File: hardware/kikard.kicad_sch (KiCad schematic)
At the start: 1 part, among them U1 NRF52840-QIAA-R

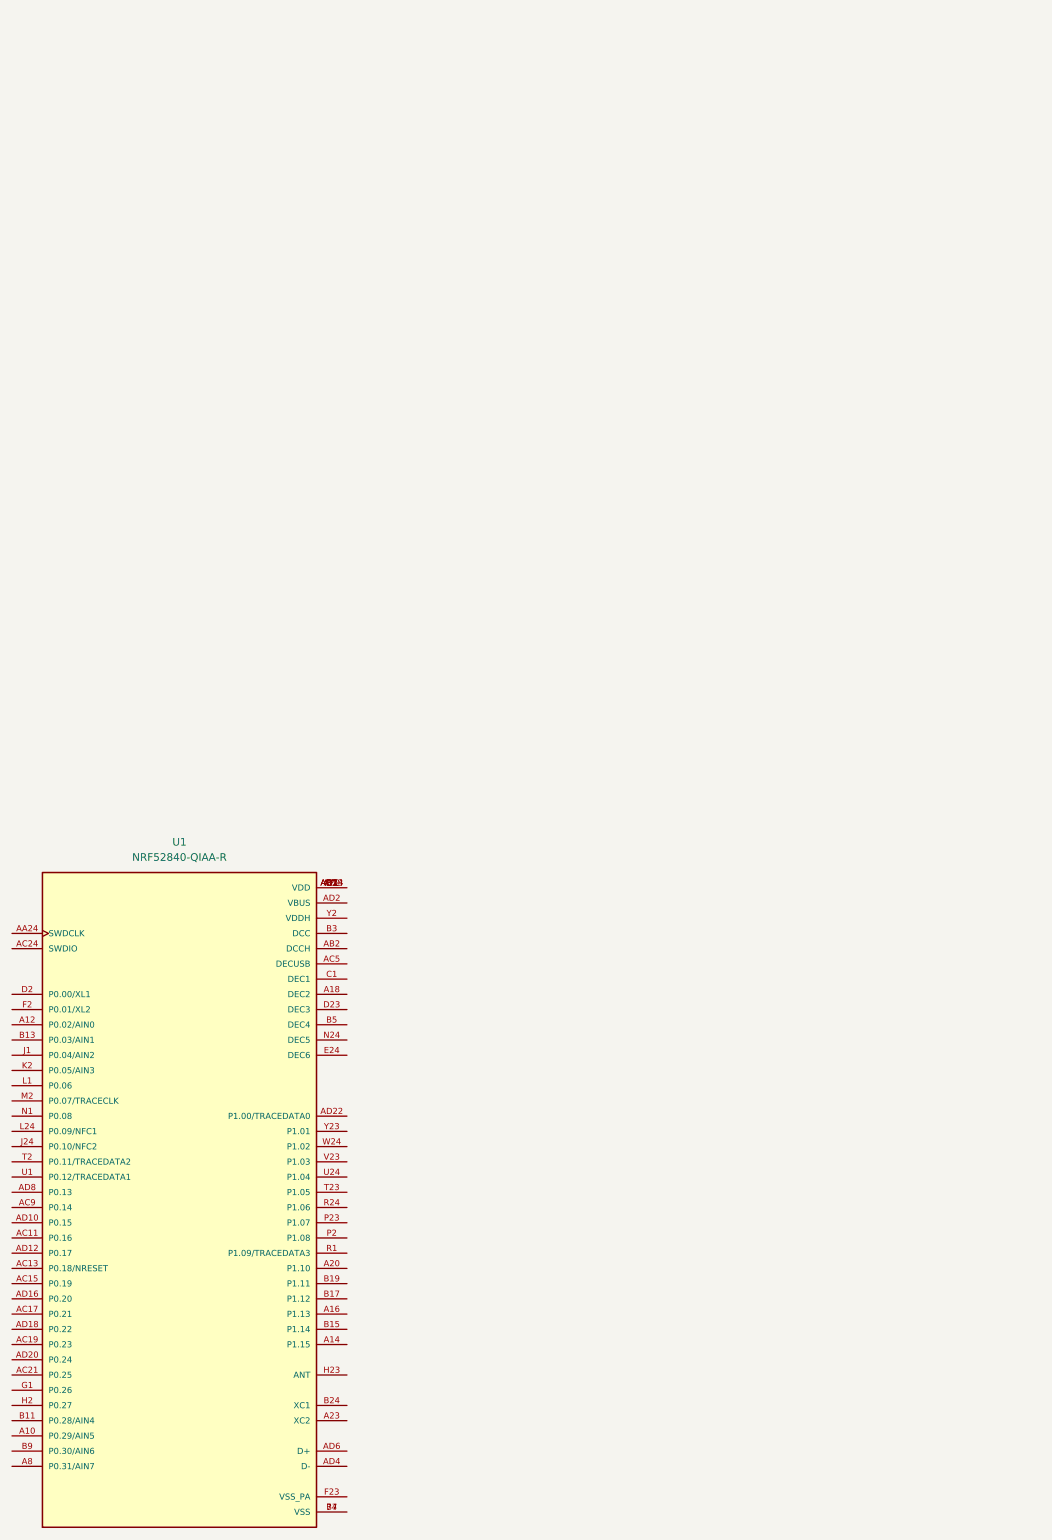
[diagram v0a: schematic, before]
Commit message: 6-4-25
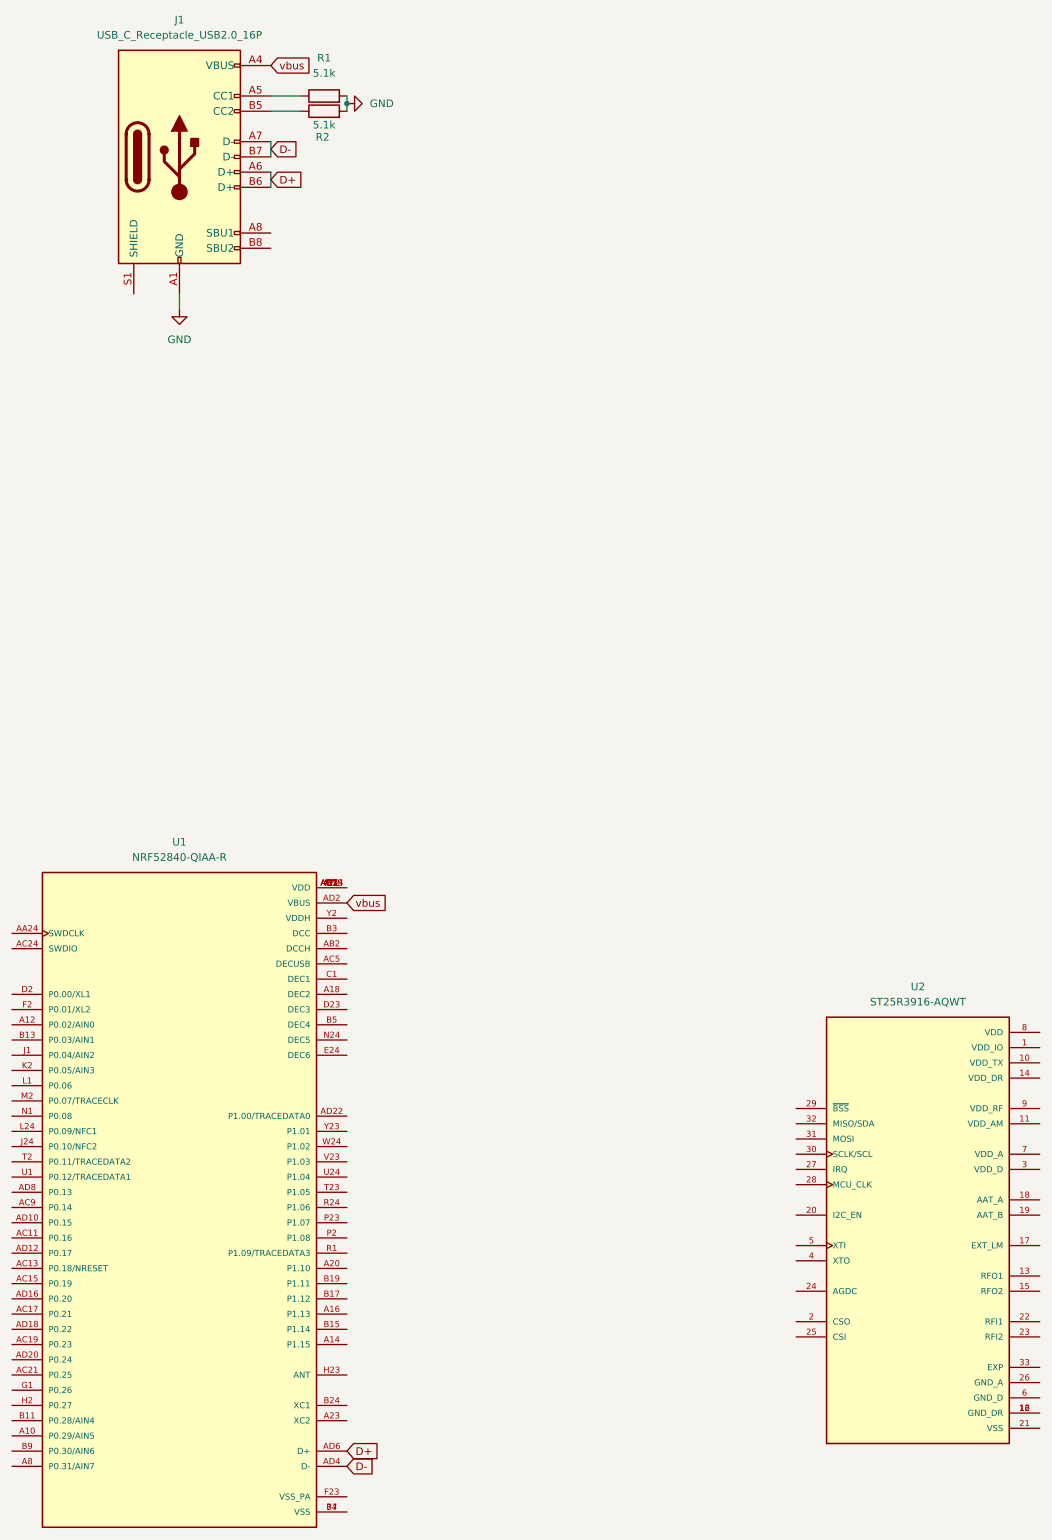
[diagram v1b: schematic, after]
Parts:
- added J1: USB_C_Receptacle_USB2.0_16P, symbol Connector:USB_C_Receptacle_USB2.0_16P
- added R1, R2: 5.1k, symbol Device:R
- added U2: ST25R3916-AQWT, ST25R3916-AQWT:QFN50P500X500X100-33N, symbol ST25R3916-AQWT:ST25R3916-AQWT
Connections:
- net vbus: now reaches U1.AD2 (VBUS)
- net vbus: now also J1.A4 (VBUS), J1.A9 (VBUS), J1.B4 (VBUS), J1.B9 (VBUS)
- net D-: now reaches U1.AD4 (D-)
- net D-: now also J1.A7 (D-), J1.B7 (D-)
- net D+: now reaches U1.AD6 (D+)
- net D+: now also J1.A6 (D+), J1.B6 (D+)
- new net: J1.A5 (CC1), R1.1
- new net: J1.B5 (CC2), R2.1
- new net: U2.12 (GND_DR), U2.16 (GND_DR)
- new net GND: J1.A1 (GND), J1.A12 (GND), J1.B1 (GND), J1.B12 (GND), R1.2, R2.2

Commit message: 6-6-25
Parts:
- added C1, C2, C3: 4.7uF, symbol Device:C
- added C10, C12, C14, C16, C18, C4, C6, C8: 10nF, symbol Device:C
- added C11: 1uF, symbol Device:C
- added C13, C15, C17, C19, C5, C7, C9: 2.2uF, symbol Device:C
- added C20, C21: 6pF, symbol Device:C
- added Y1: XRCGB27M120F3M00R0, symbol Device:Crystal_GND2
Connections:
- net vbus is gone; now on net vusb: J1.A4 (VBUS), J1.A9 (VBUS), J1.B4 (VBUS), J1.B9 (VBUS), U1.AD2 (VBUS)
- net GND: now also J1.S1 (SHIELD), U1.74 (VSS), U1.B7 (VSS), U2.12 (GND_DR), U2.16 (GND_DR), U2.20 (I2C_EN), U2.21 (VSS), U2.26 (GND_A), U2.33 (EXP), U2.6 (GND_D), C1.1, C10.1, C11.1, C12.1, C13.1, C14.1, C15.1, C16.1, C17.1, C18.1, C19.1, C2.1, C20.1, C21.1, C3.2, C4.1, C5.1, C6.1, C7.1, C8.1, C9.1, Y1.2
- net VDD3.3v: now reaches U2.1 (VDD_IO)
- net VDD3.3v: now also U1.A22 (VDD), U1.AD14 (VDD), U1.AD23 (VDD), U1.B1 (VDD), U1.W1 (VDD), C2.2, C6.2, C7.2
- net vusb: now reaches U2.10 (VDD_TX)
- net vusb: now also U2.8 (VDD), C3.1, C4.2, C5.2, C8.2, C9.2
- net at U2.11 (VDD_AM): now also C14.2, C15.2
- net at U2.14 (VDD_DR): now also U2.9 (VDD_RF), C12.2, C13.2
- net at U2.24 (AGDC): now also C10.2, C11.2
- net IRQ: now reaches U2.27 (IRQ)
- net IRQ: now also U1.N1 (P0.08)
- net CS: now reaches U2.29 (~{BSS})
- net CS: now also U1.M2 (P0.07/TRACECLK)
- net at U2.3 (VDD_D): now also C18.2, C19.2
- net SCLK: now reaches U2.30 (SCLK/SCL)
- net SCLK: now also U1.J1 (P0.04/AIN2)
- net MOSI: now reaches U2.31 (MOSI)
- net MOSI: now also U1.K2 (P0.05/AIN3)
- net MISO: now reaches U2.32 (MISO/SDA)
- net MISO: now also U1.L1 (P0.06)
- net at U2.4 (XTO): now also C21.2, Y1.3
- net at U2.5 (XTI): now also C20.2, Y1.1
- net at U2.7 (VDD_A): now also C16.2, C17.2
- net at U1.AC5 (DECUSB): now also C1.2
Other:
- moved on the sheet: U2

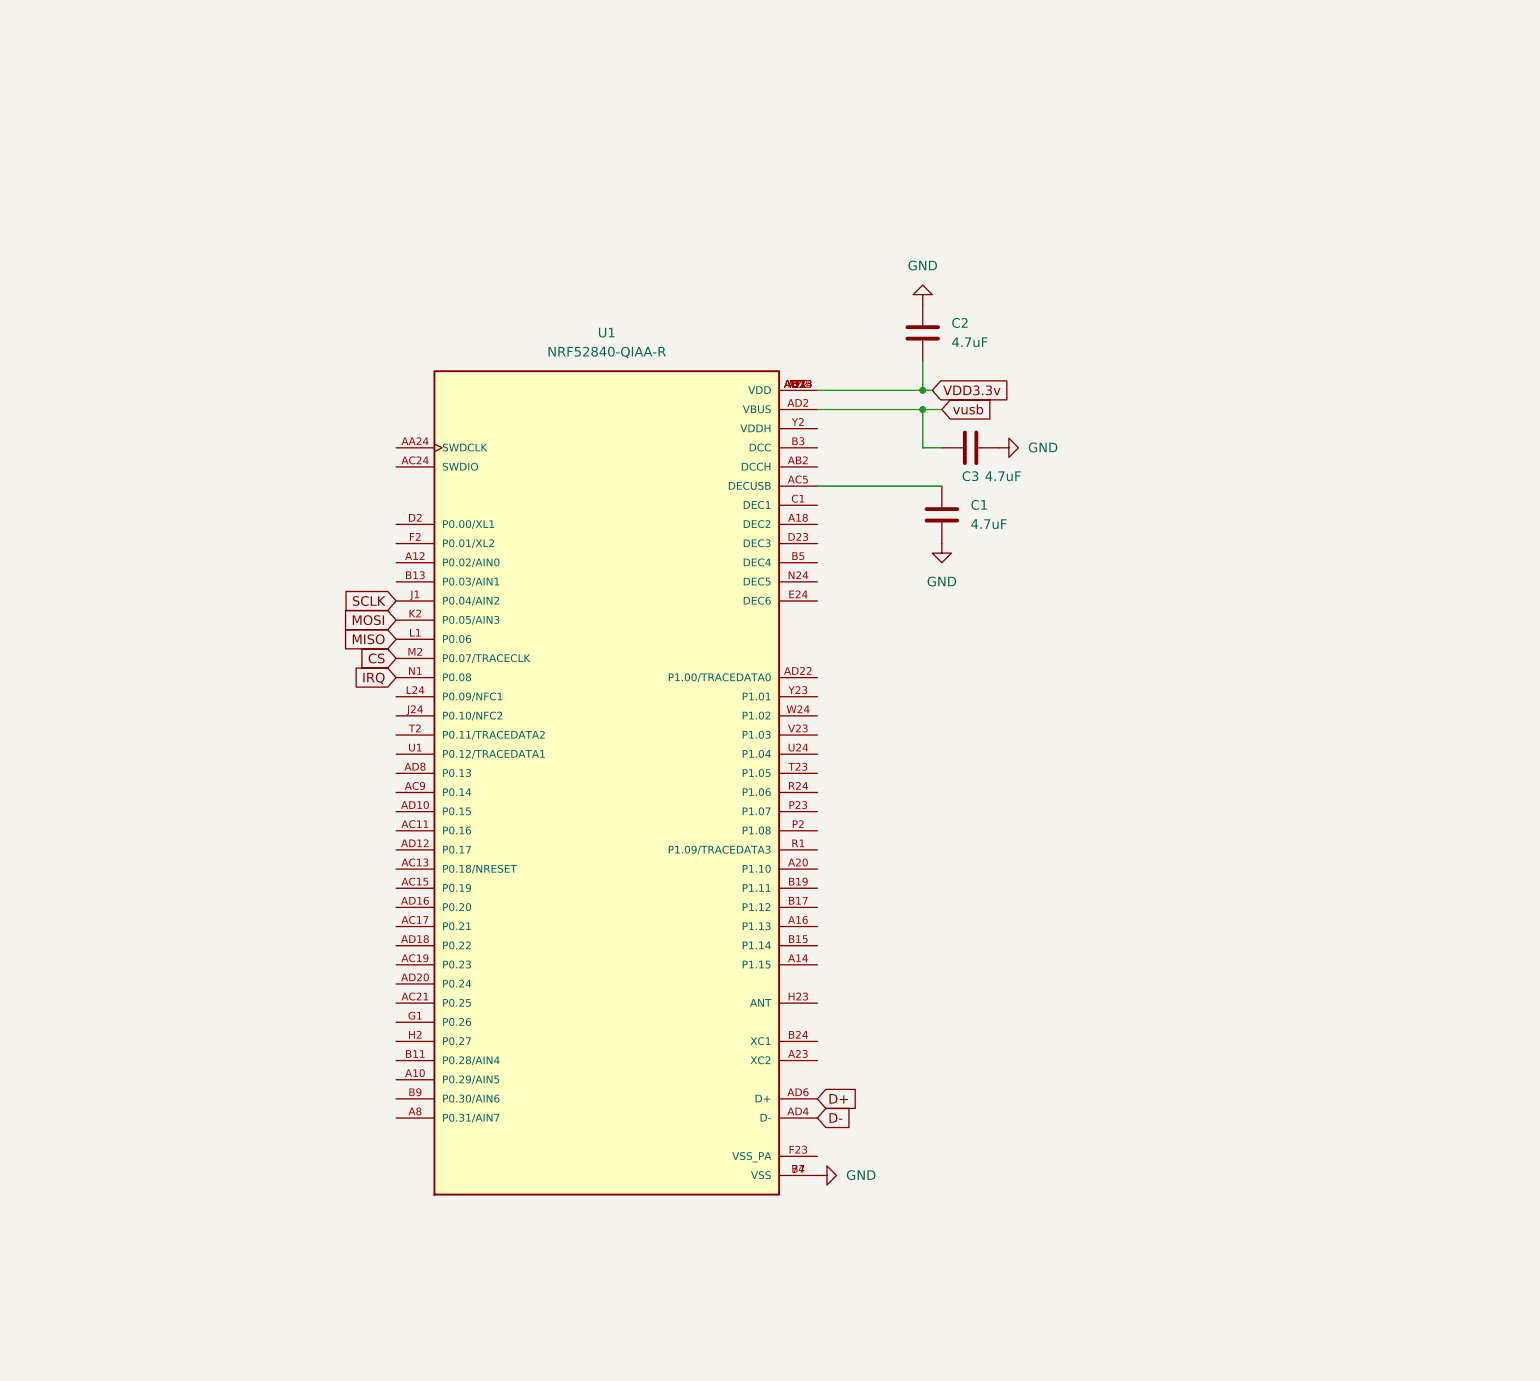
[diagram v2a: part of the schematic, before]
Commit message: 6-29-25
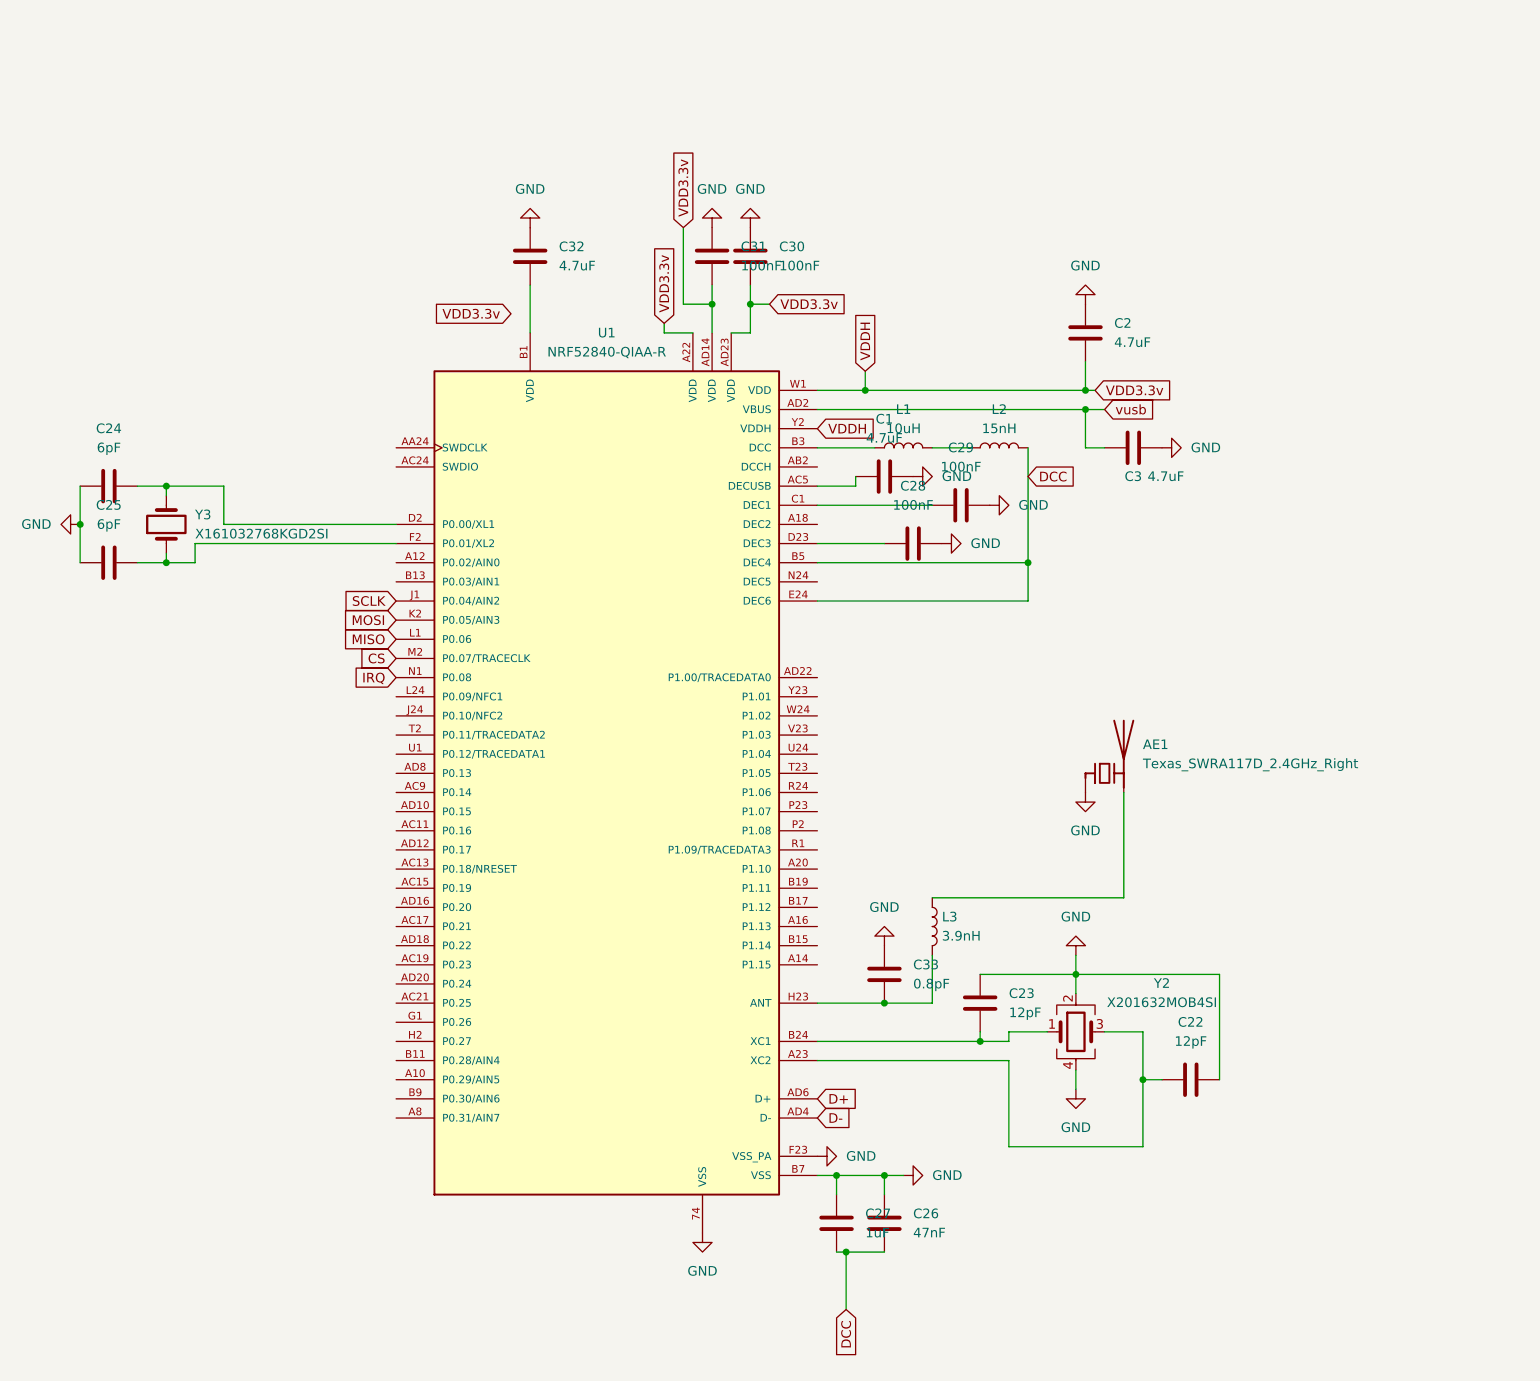
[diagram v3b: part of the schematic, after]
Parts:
- added AE1: Texas_SWRA117D_2.4GHz_Right, extra-symbols-footprints:Texas_SWRA117D_2.4GHz_Right, symbol Device:Antenna_Chip
- added C22, C23: 12pF, symbol Device:C
- added C24, C25: 6pF, symbol Device:C
- added C26: 47nF, symbol Device:C
- added C27: 1uF, symbol Device:C
- added C28, C29, C30, C31: 100nF, symbol Device:C
- added C32: 4.7uF, symbol Device:C
- added C33: 0.8pF, symbol Device:C
- added L1: 10uH, symbol Device:L
- added L2: 15nH, symbol Device:L
- added L3: 3.9nH, symbol Device:L
- added Y2: X201632MOB4SI, symbol Device:Crystal_GND24
- added Y3: X161032768KGD2SI, symbol Device:Crystal
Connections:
- net GND: now also U1.F23 (VSS_PA), AE1.1 (FEED), C22.2, C23.2, C24.1, C25.1, C26.1, C27.1, C28.2, C29.2, C30.1, C31.1, C32.1, C33.1, Y2.2, Y2.4
- net VDD3.3v: now also U1.Y2 (VDDH), C30.2, C31.2; no longer U1.B1 (VDD)
- net at U1.A23 (XC2): now also C22.1, Y2.3
- net at U1.B24 (XC1): now also C23.1, Y2.1
- net at U1.B3 (DCC): now also L1.1
- net DCC: now reaches U1.B5 (DEC4)
- net DCC: now also U1.E24 (DEC6), C26.2, C27.2, L2.2
- net at U1.C1 (DEC1): now also C29.1
- net at U1.D2 (P0.00/XL1): now also C24.2, Y3.2
- net at U1.D23 (DEC3): now also C28.1
- net at U1.F2 (P0.01/XL2): now also C25.2, Y3.1
- net at U1.H23 (ANT): now also C33.2, L3.2
- new net: C32.2, U1.B1 (VDD)
- new net: AE1.2 (PCB_Trace), L3.1
- new net: L1.2, L2.1
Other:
- moved on the sheet: C1, C2, C3
